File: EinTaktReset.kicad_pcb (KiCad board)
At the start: 2 copper layers, 100 x 160 mm, 68 parts, among them J1 Conn_01x02, J2 Conn_01x03, J3 Conn_01x03, J4 Conn_01x03, J5 Conn_01x02, J6 Conn_01x02, P1 CONN_02X10, P4 CONN_02X10, SW1 Digitast, SW10 SPST, SW11 SPST, SW12 SPST, SW13 SPST, SW2 Digitast, SW3 SW_SPDT, SW4 SW_SPDT, SW5 SPST, SW6 SW_SPDT, SW7 SPST, SW8 SPST, SW9 SPST, U1 74132, U2 74540, U3 74HCT541_PWR, U4 7432, U5 7400, U6 74HC4046

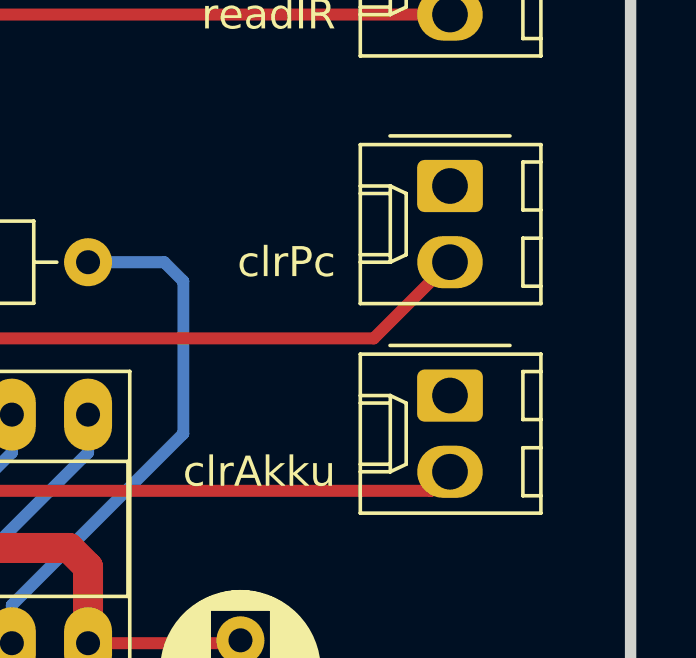
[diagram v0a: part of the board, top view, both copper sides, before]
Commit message: viele kleine Änderungen
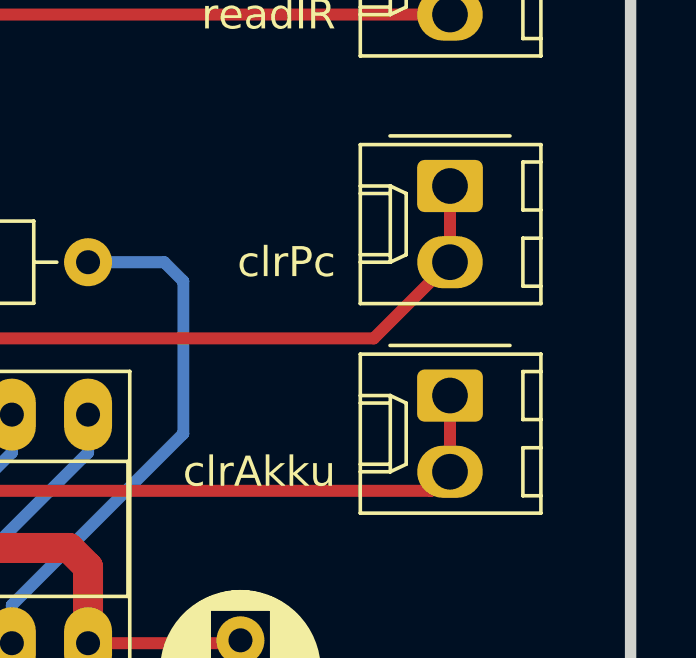
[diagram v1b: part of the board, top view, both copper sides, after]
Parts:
- U3: value 74HCT541_PWR -> 74HC541
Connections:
- net auto renamed ~auto
- net clrMPC renamed ~clrMPC
- net en-ln1 renamed ~en-ln1
- net en-ln2 renamed ~en-ln2
- net enAkku renamed ~enAkku
- net loadIR renamed ~loadIR
- J5 pad 1: Net-(J5-Pad1) -> clrPC
- J6 pad 1: Net-(J6-Pad1) -> clrAkku
- P1 pad 11: /a4 -> /a3
- P1 pad 13: /a5 -> /a2
- P1 pad 15: /a6 -> /a1
- P1 pad 17: /a7 -> /a0
- P1 pad 3: /a0 -> /a7
- P1 pad 5: /a1 -> /a6
- P1 pad 7: /a2 -> /a5
- P1 pad 9: /a3 -> /a4
- P4 pad 11: /a4 -> /a3
- P4 pad 13: /a5 -> /a2
- P4 pad 15: /a6 -> /a1
- P4 pad 17: /a7 -> /a0
- P4 pad 3: /a0 -> /a7
- P4 pad 5: /a1 -> /a6
- P4 pad 7: /a2 -> /a5
- P4 pad 9: /a3 -> /a4
- U3 pad 11: /a7 -> /a0
- U3 pad 12: /a6 -> /a1
- U3 pad 13: /a5 -> /a2
- U3 pad 14: /a4 -> /a3
- U3 pad 15: /a3 -> /a4
- U3 pad 16: /a2 -> /a5
- U3 pad 17: /a1 -> /a6
- U3 pad 18: /a0 -> /a7
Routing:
- net /a7: track 97.4 -> 106.4 mm, vias 0 -> 1
- net /a0: track 106.4 -> 97.4 mm, vias 1 -> 0
- net /a6: track 98.2 -> 105.7 mm
- net /a1: track 105.7 -> 98.2 mm
- net /a5: track 99.5 -> 103.7 mm
- net /a2: track 103.7 -> 99.5 mm
- net clrPC: track 25.4 -> 28.0 mm
- net clrAkku: track 22.1 -> 24.7 mm
- net /a4: track 100.9 -> 102.3 mm
- net /a3: track 102.3 -> 100.9 mm

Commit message: Netze umbenannt
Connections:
- net ~enAkku renamed ~writeAccu
- net ~loadIR renamed ~readIR
